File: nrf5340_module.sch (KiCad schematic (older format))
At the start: 42 parts, among them J1 U.FL_A-1JB, U1 nrf5340, Y1 32.768kHz, Y2 32MHz

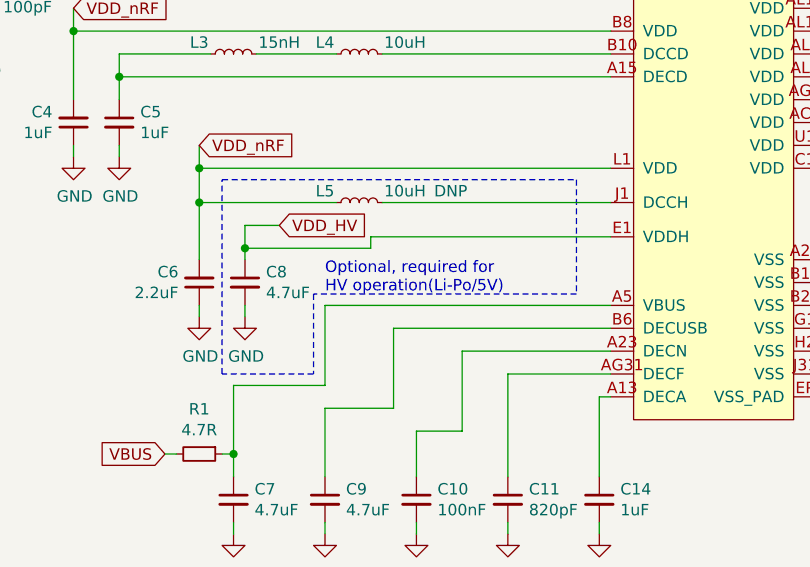
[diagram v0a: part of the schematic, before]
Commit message: update
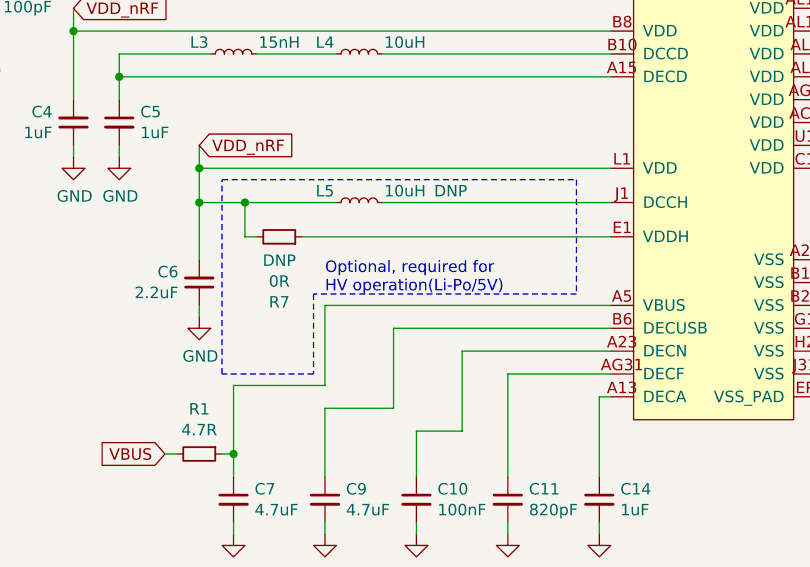
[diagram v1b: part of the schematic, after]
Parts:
- removed C8: 4.7uF, Capacitor_SMD:C_0603_1608Metric, symbol Device:C_Small
- added R7: 0R, Resistor_SMD:R_0603_1608Metric, symbol Device:R_Small
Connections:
- net VDD_nRF: now also R7.2
- net VDD_HV: no longer names the net of U1.E1 (VDDH)
- net VDD_HV: now also R7.1
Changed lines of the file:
@@
 EESchema Schematic File Version 4
-LIBS:nrf5340_module-cache
 EELAYER 30 0
 EELAYER END
@@
 Title "nrf5340_module"
 Date "2019-11-17"
-Rev "1.0.0"
+Rev "1.0"
 Comp ""
 Comment1 ""
@@
 $EndComp
 $Comp
-L Device:C_Small C8
-U 1 1 5DDBE086
-P 5350 2700
-F 0 "C8" H 5442 2746 50  0000 L CNN
-F 1 "4.7uF" H 5442 2655 50  0000 L CNN
-F 2 "Capacitor_SMD:C_0603_1608Metric" H 5350 2700 50  0001 C CNN
-F 3 "~" H 5350 2700 50  0001 C CNN
-	1    5350 2700
-	1    0    0    -1
-$EndComp
-$Comp
 L power:GND #PWR0106
 U 1 1 5DDBE08C
@@
 	1    0    0    -1
 $EndComp
-$Comp
-L power:GND #PWR0107
-U 1 1 5DDBE092
-P 5350 2850
-F 0 "#PWR0107" H 5350 2600 50  0001 C CNN
-F 1 "GND" H 5355 2677 50  0000 C CNN
-F 2 "" H 5350 2850 50  0001 C CNN
-F 3 "" H 5350 2850 50  0001 C CNN
-	1    5350 2850
-	1    0    0    -1
-$EndComp
-Wire Wire Line
-	5350 2800 5350 2850
 Wire Wire Line
 	5150 2800 5150 2850
@@
 	5950 2350 6950 2350
 Wire Wire Line
-	5750 2350 5150 2350
+	5750 2350 5350 2350
 Connection ~ 5150 2350
-Text GLabel 5500 2450 2    50   Input ~ 0
-VDD_HV
-Wire Wire Line
-	5500 2450 5350 2450
-Wire Wire Line
-	5350 2450 5350 2550
-Wire Wire Line
-	5350 2550 5900 2550
-Wire Wire Line
-	5900 2550 5900 2500
-Wire Wire Line
-	5900 2500 6950 2500
-Connection ~ 5350 2550
-Wire Wire Line
-	5350 2550 5350 2600
 Wire Wire Line
 	5150 2350 5150 2600
@@
 NoConn ~ 3850 7450
 NoConn ~ 1500 5500
+$Comp
+L Device:R_Small R7
+U 1 1 602574E0
+P 5500 2500
+F 0 "R7" V 5214 2500 50  0000 C CNN
+F 1 "0R" V 5305 2500 50  0000 C CNN
+F 2 "Resistor_SMD:R_0603_1608Metric" H 5500 2500 50  0001 C CNN
+F 3 "~" H 5500 2500 50  0001 C CNN
+F 4 "DNP" V 5396 2500 50  0000 C CNN "DNP"
+	1    5500 2500
+	0    1    -1   0
+$EndComp
+Wire Wire Line
+	5600 2500 6950 2500
+Wire Wire Line
+	5400 2500 5350 2500
+Wire Wire Line
+	5350 2500 5350 2350
+Connection ~ 5350 2350
+Wire Wire Line
+	5350 2350 5150 2350
 $EndSCHEMATC
